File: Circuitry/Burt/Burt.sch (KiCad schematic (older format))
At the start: 40 parts, among them J1 Conn_01x20, J2 Conn_01x08_Female, M1 Motor_DC, Q1 SSM6N58NU, Q2 SSM6N58NU, Q3 SSM6N58NU, Q4 SSM6N58NU, Q5 SSM6N58NU, U1 MCP9701A, U2 A3908, U3 MCP73831-DFN, U4 74HC595

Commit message: Did lt surge
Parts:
- J1: Part URL (none) -> https://www.digikey.com/product-detail/en/amphenol-icc-fci/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
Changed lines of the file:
@@
 F 2 "Custom:62674-201121ALF" H 5025 5275 50  0001 C CNN
 F 3 "~" H 5025 5275 50  0001 C CNN
+F 4 "https://www.digikey.com/product-detail/en/amphenol-icc-fci/62674-201121ALF/609-1207-1-ND/1003043" H 5025 5275 50  0001 C CNN "Part URL"
 	1    5025 5275
 	1    0    0    -1
@@
 NoConn ~ 4825 6275
 $Comp
-L power:+BATT #PWR?
+L power:+BATT #PWR0140
 U 1 1 5D659F24
 P 6225 1075
-F 0 "#PWR?" H 6225 925 50  0001 C CNN
+F 0 "#PWR0140" H 6225 925 50  0001 C CNN
 F 1 "+BATT" H 6240 1248 50  0000 C CNN
 F 2 "" H 6225 1075 50  0001 C CNN

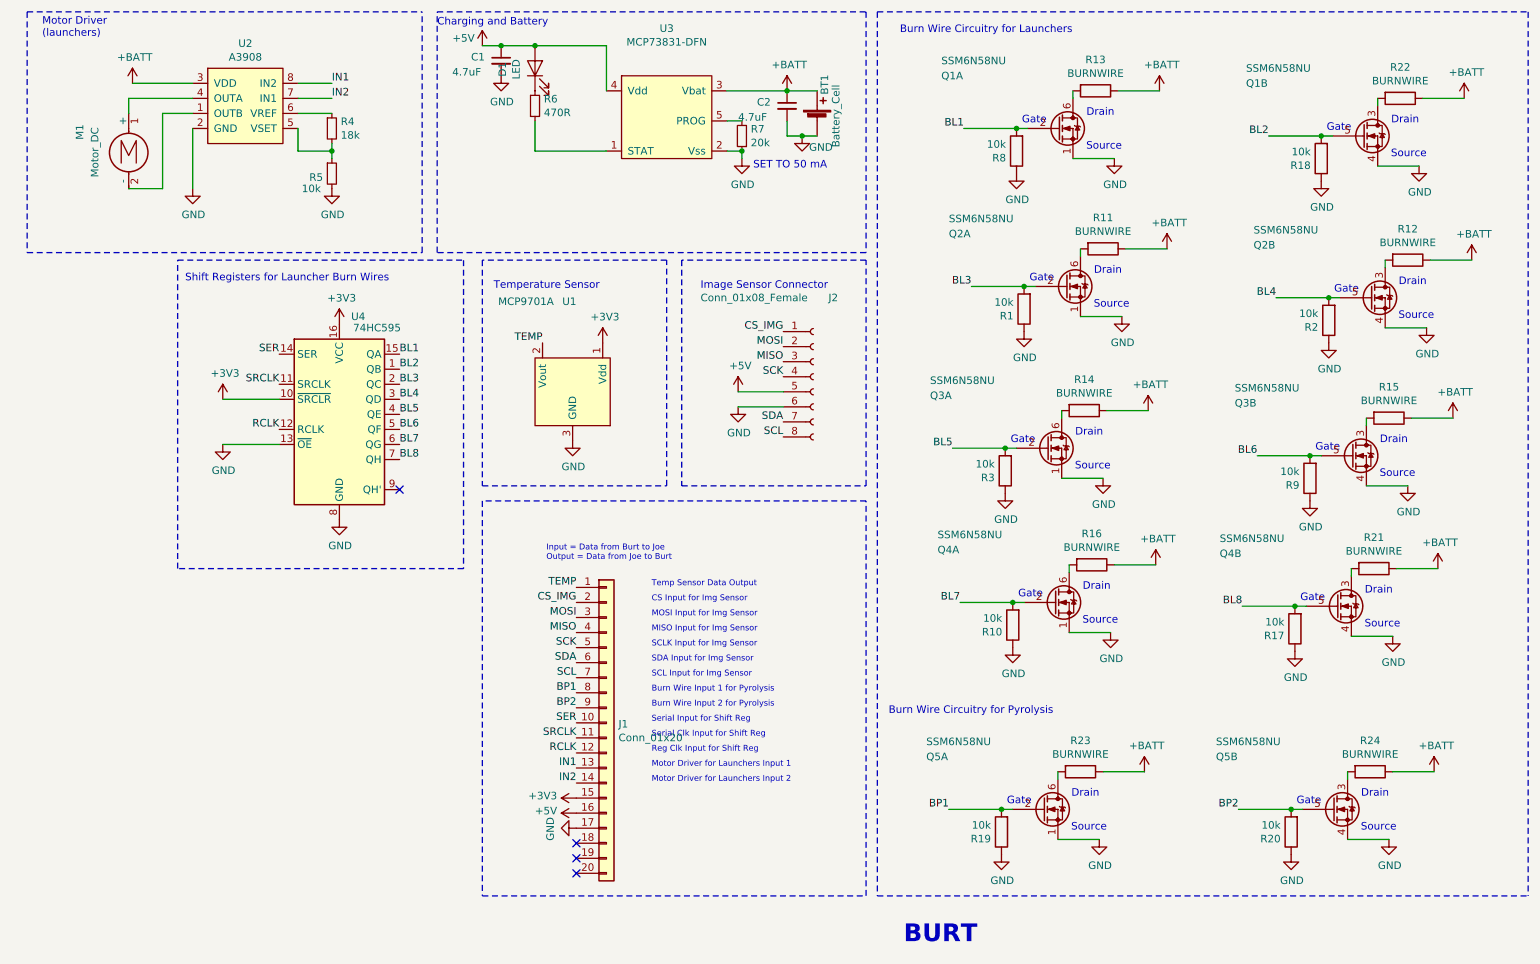
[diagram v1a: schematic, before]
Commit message: Finshed lt surge layout
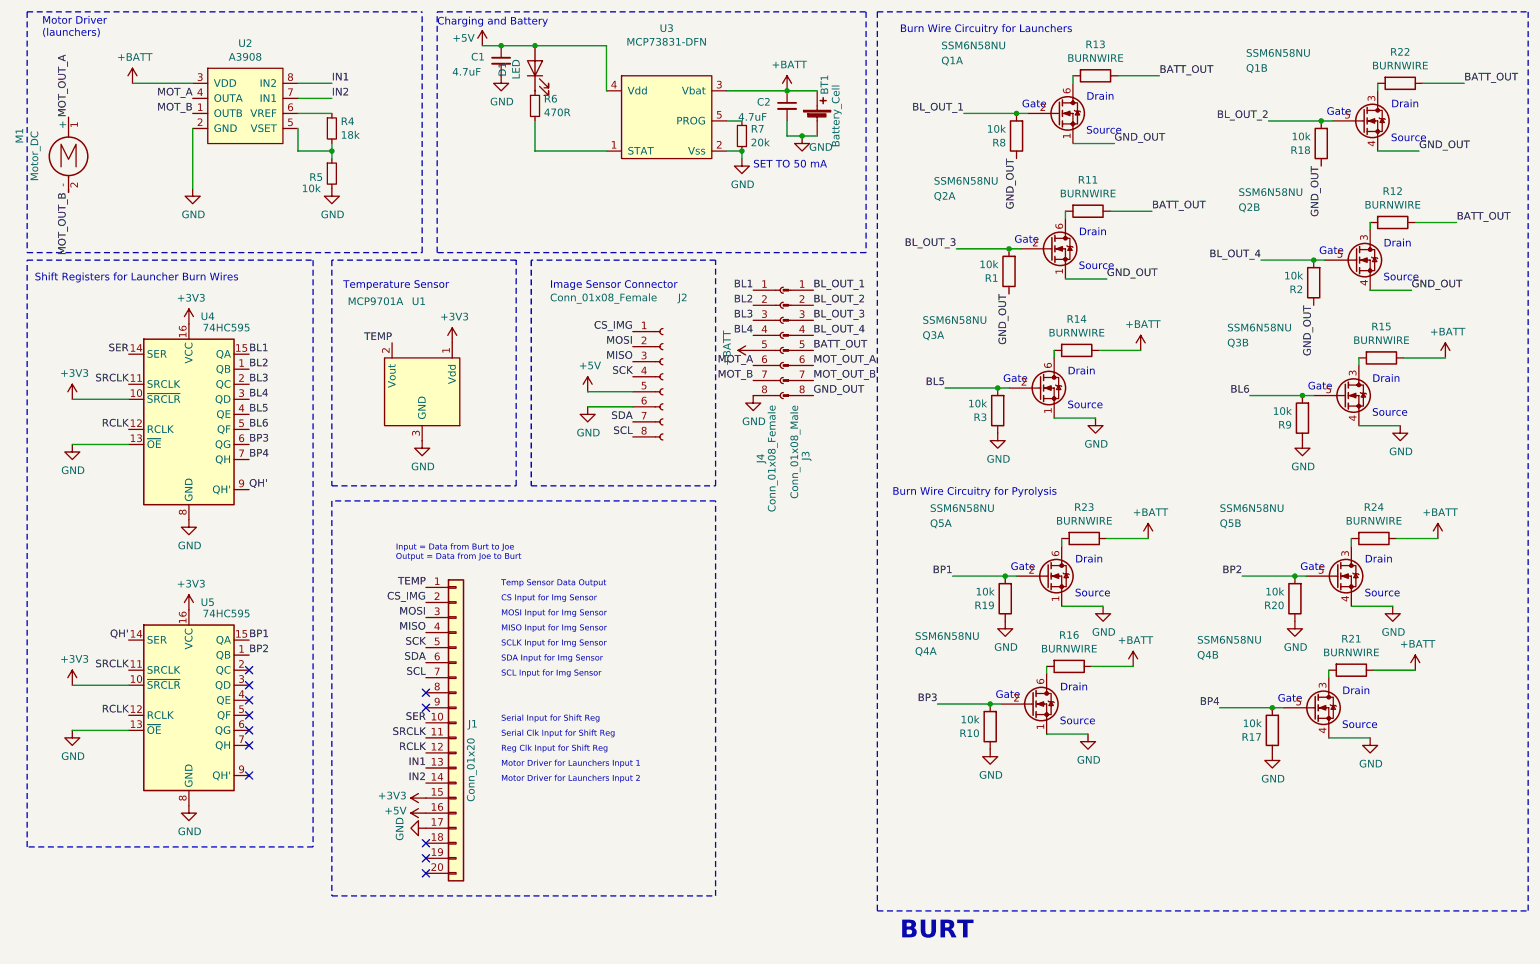
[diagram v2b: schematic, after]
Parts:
- added J3: Conn_01x08_Male, Connector_PinHeader_1.00mm:PinHeader_1x08_P1.00mm_Vertical, symbol Connector:Conn_01x08_Male
- added J4: Conn_01x08_Female, Connector_PinHeader_1.00mm:PinHeader_1x08_P1.00mm_Vertical, symbol Connector:Conn_01x08_Female
- added U5: 74HC595, Package_SO:SOIC-16_3.9x9.9mm_P1.27mm, symbol 74xx:74HC595
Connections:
- net +3V3: now also U5.10 (~SRCLR), U5.16 (VCC)
- net +BATT: now also J4.5 (Pin_5); no longer R11.1, R12.1, R13.1, R22.1
- net BL1: now also J4.1 (Pin_1); no longer Q1.2 (G), R8.2
- net BL2: now also J4.2 (Pin_2); no longer Q1.5 (G), R18.2
- net BL3: now also J4.3 (Pin_3); no longer Q2.2 (G), R1.2
- net BL4: now also J4.4 (Pin_4); no longer Q2.5 (G), R2.2
- net BP1: now also U5.15 (QA); no longer J1.8 (Pin_8)
- net BP2: now also U5.1 (QB); no longer J1.9 (Pin_9)
- net GND: now also J4.8 (Pin_8), U5.13 (~OE), U5.8 (GND); no longer Q1.1 (S), Q1.4 (S), Q2.1 (S), Q2.4 (S), R1.1, R18.1, R2.1, R8.1
- net RCLK: now also U5.12 (RCLK)
- net SRCLK: now also U5.11 (SRCLK)
- net QH': now reaches U4.9 (QH')
- net QH': now also U5.14 (SER)
- net MOT_A: now reaches U2.4 (OUTA)
- net MOT_A: now also J4.6 (Pin_6); no longer M1.1 (+)
- net MOT_B: now reaches U2.1 (OUTB)
- net MOT_B: now also J4.7 (Pin_7); no longer M1.2 (-)
- net BL7 renamed BP3
- net BL8 renamed BP4
- new net BATT_OUT: J3.5 (Pin_5), R11.1, R12.1, R13.1, R22.1
- new net BL_OUT_1: J3.1 (Pin_1), Q1.2 (G), R8.2
- new net BL_OUT_2: J3.2 (Pin_2), Q1.5 (G), R18.2
- new net BL_OUT_3: J3.3 (Pin_3), Q2.2 (G), R1.2
- new net BL_OUT_4: J3.4 (Pin_4), Q2.5 (G), R2.2
- new net GND_OUT: J3.8 (Pin_8), Q1.1 (S), Q1.4 (S), Q2.1 (S), Q2.4 (S), R1.1, R18.1, R2.1, R8.1
- new net MOT_OUT_A: J3.6 (Pin_6), M1.1 (+)
- new net MOT_OUT_B: J3.7 (Pin_7), M1.2 (-)
- no-connect marks 4 -> 12
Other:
- note removed: "Burn Wire Input 1 for Pyrolysis"
- note removed: "Burn Wire Input 2 for Pyrolysis"
- moved on the sheet: J1, J2, M1, Q1A, Q1B, Q2A, Q2B, Q3A, Q3B, Q4A, Q4B, Q5A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
